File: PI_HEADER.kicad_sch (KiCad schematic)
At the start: 6 parts, among them J14 PRT-14017, J6 ADC_CONN

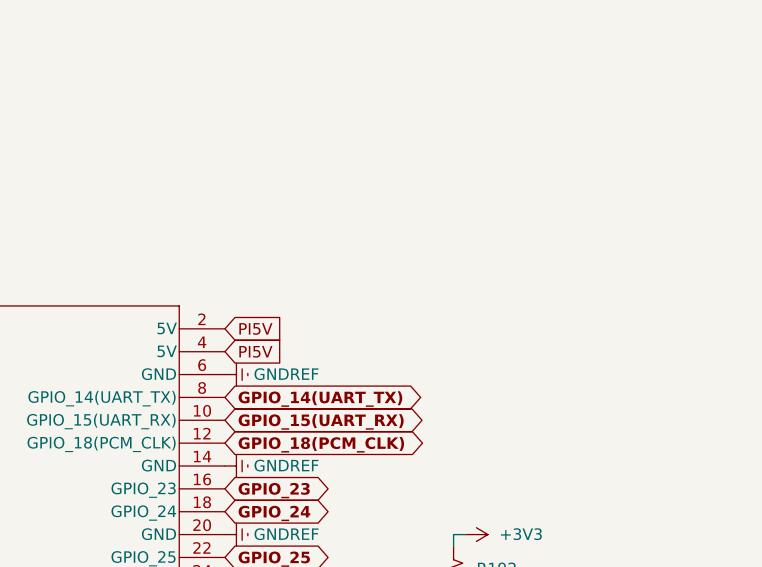
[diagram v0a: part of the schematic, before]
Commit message: ready for manufacturing
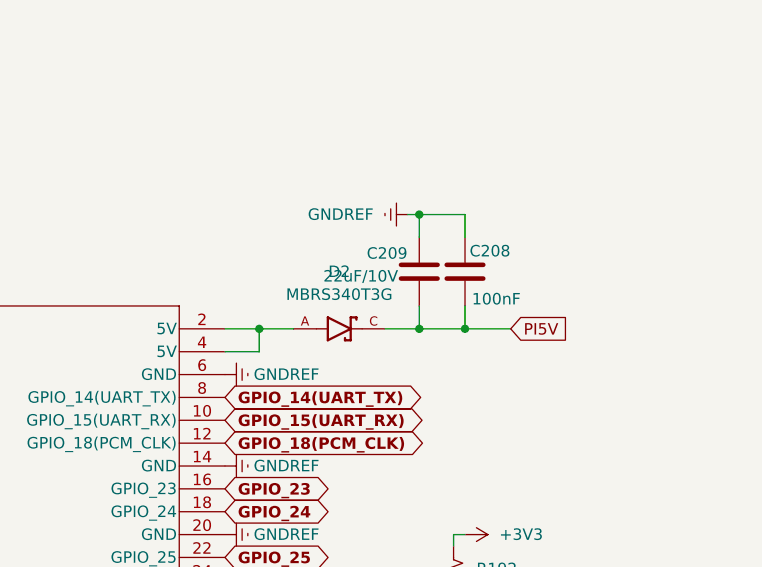
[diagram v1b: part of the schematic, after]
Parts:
- added C208: 100nF, footprints:C_0201_0603Metric, symbol Device:C
- added C209: 22uF/10V, footprints:C_0805, symbol Device:C
- added D2: MBRS340T3G, footprints:DIOM7959X261N, symbol MBRS340T3G:MBRS340T3G
- J14, J6: LCSC PN digi/mouser -> (none)
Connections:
- net GNDREF: now also C208.1, C209.1
- net PI5V: now also C208.2, C209.2, D2.C; no longer J14.2 (5V), J14.4 (5V)
- new net: D2.A, J14.2 (5V), J14.4 (5V)
